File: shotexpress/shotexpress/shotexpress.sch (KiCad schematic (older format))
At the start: 16 parts

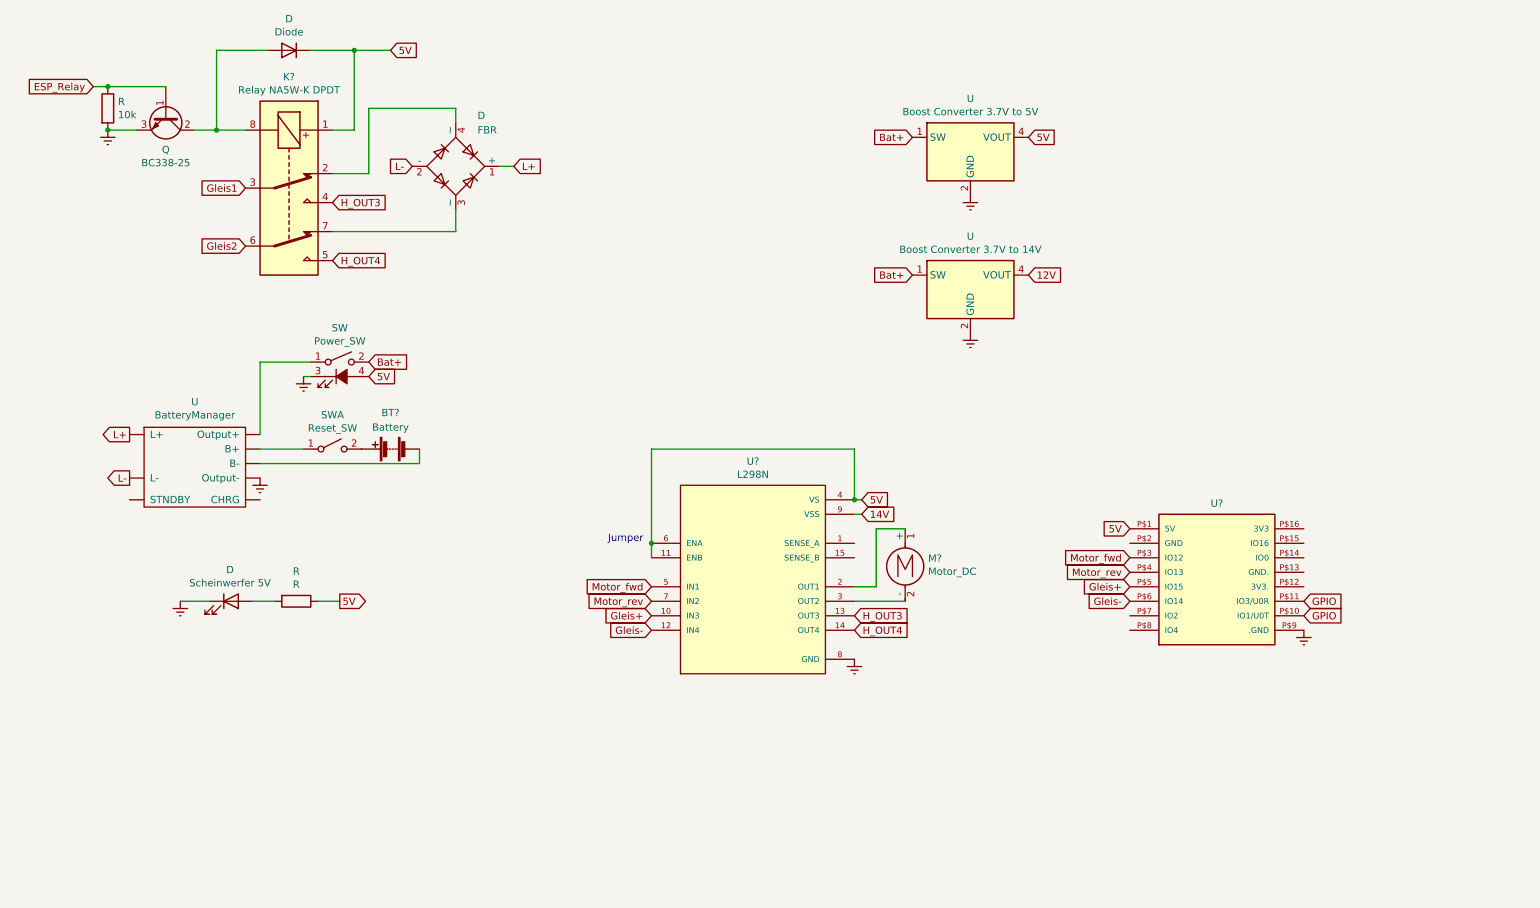
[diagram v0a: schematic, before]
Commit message: Correct kicad scheme
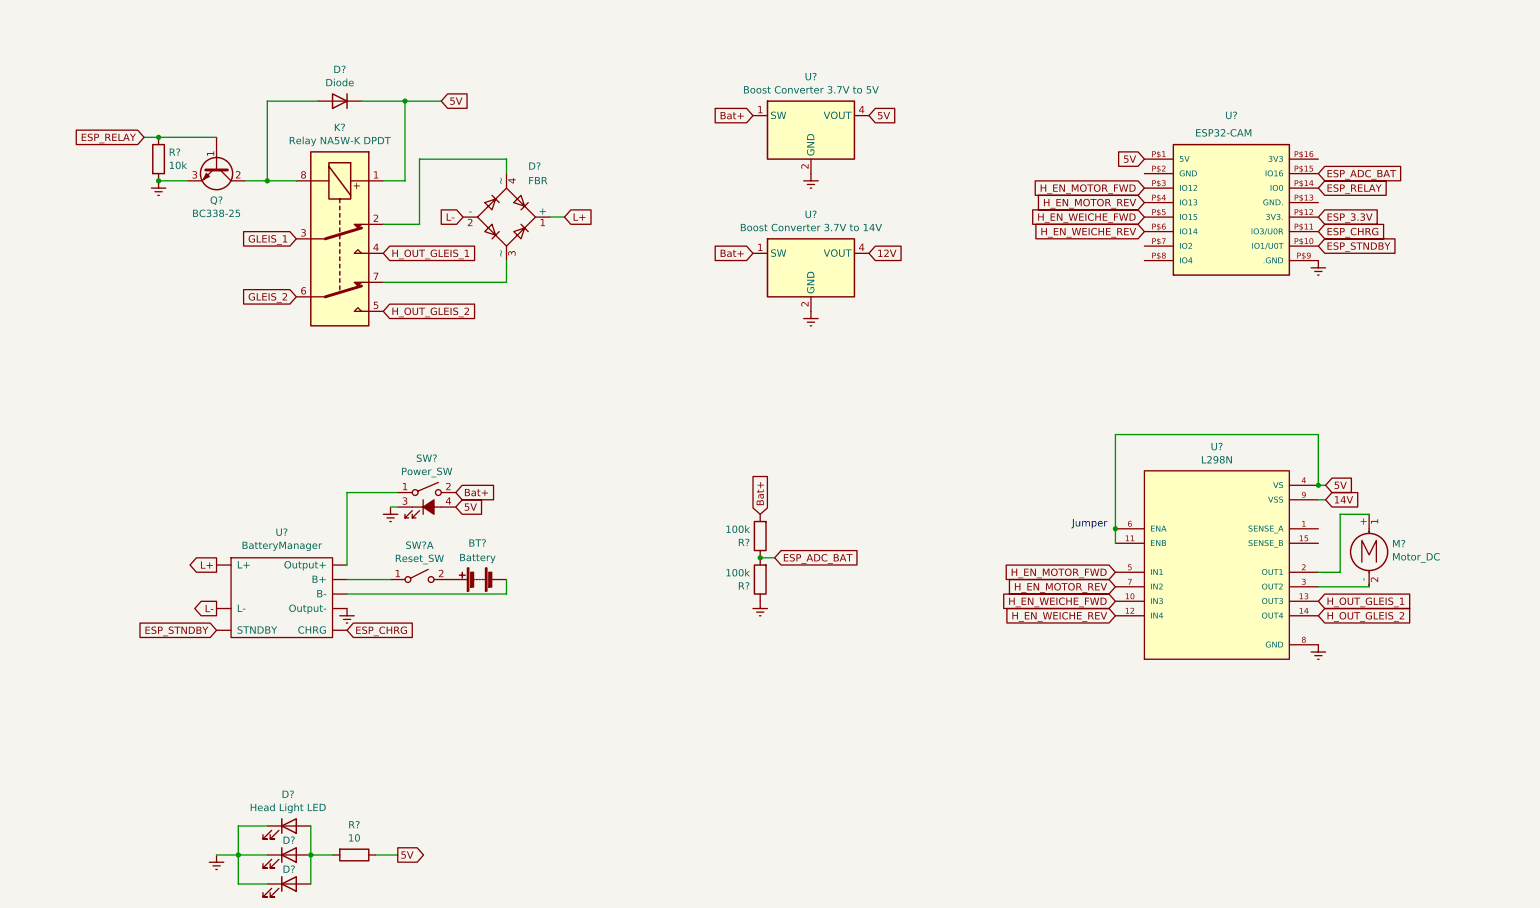
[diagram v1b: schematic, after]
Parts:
- added D? (x2): Scheinwerfer 5V, symbol Device:LED
- added R? (x2): 100k, symbol Device:R
- D?: renamed from D; value Scheinwerfer 5V -> Head Light LED
- R?: renamed from R; value R -> 10
- renumbered D to D?, Q to Q?, R to R?, SW to SW?, U to U?
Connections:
- net ESP_Relay is gone; now on net ESP_RELAY: Q?.1 (B), R?.1
- net Bat+: now also R?.2
- net Earth: now also D?.1 (K), D?.1 (K), R?.1
- net ESP_3.3V: now reaches U?.P$12 (3V3.)
- net ESP_RELAY: now reaches U?.P$14 (IO0)
- net ESP_ADC_BAT: now reaches U?.P$15 (IO16)
- net ESP_ADC_BAT: now also R?.1, R?.2
- net at D?.2 (A), R?.2: now also D?.2 (A), D?.2 (A)
- net GPIO renamed ESP_CHRG
- net ESP_CHRG: now also U?.~ (STNDBY); no longer U?.P$10 (IO1/U0T)
- net Gleis+ renamed H_EN_WEICHE_FWD
- net Gleis- renamed H_EN_WEICHE_REV
- net Gleis1 renamed GLEIS_1
- net Gleis2 renamed GLEIS_2
- net H_OUT3 renamed H_OUT_GLEIS_1
- net H_OUT4 renamed H_OUT_GLEIS_2
- net Motor_fwd renamed H_EN_MOTOR_FWD
- net Motor_rev renamed H_EN_MOTOR_REV
- new net ESP_STNDBY: U?.P$10 (IO1/U0T), U?.~ (STNDBY)
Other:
- moved on the sheet: BT?, D?, K?, M?, Q?, R?, SW?, SW?A, U?

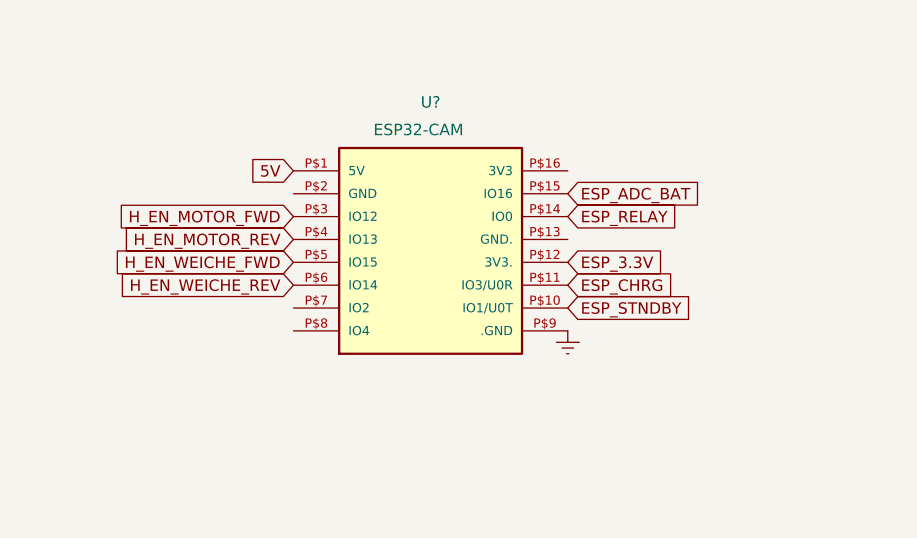
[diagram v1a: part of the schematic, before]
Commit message: Complete Kicad files
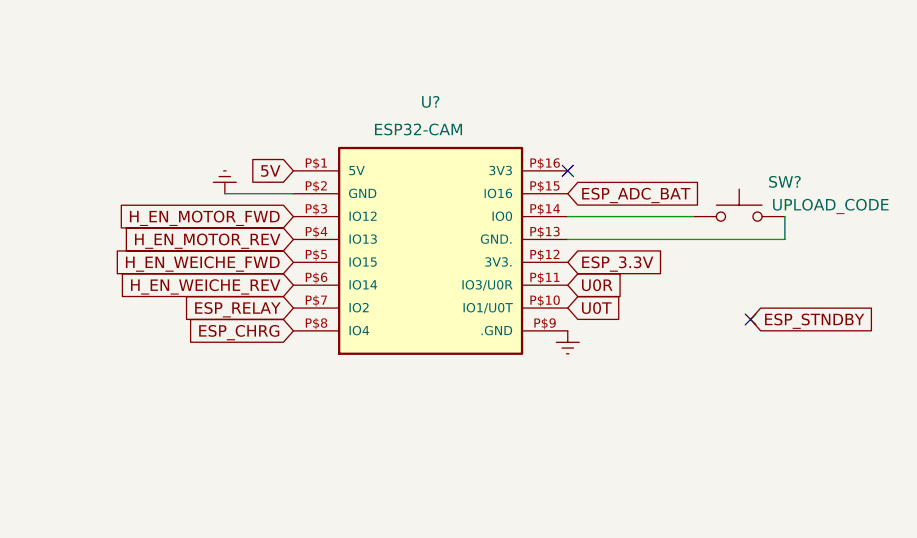
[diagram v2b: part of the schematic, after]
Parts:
- added SW?: UPLOAD_CODE, symbol Switch:SW_MEC_5G
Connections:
- net ESP_CHRG: now also U?.P$8 (IO4); no longer U?.P$11 (IO3/U0R)
- net ESP_RELAY: now also U?.P$7 (IO2); no longer U?.P$14 (IO0)
- net ESP_STNDBY: no longer U?.P$10 (IO1/U0T)
- net Earth: now also U?.P$2 (GND)
- net at U?.P$13 (GND.): now also SW?.3 (B), SW?.4 (B)
- new net: SW?.1 (A), SW?.2 (A), U?.P$14 (IO0)
- new net U0R: U?.P$11 (IO3/U0R)
- new net U0T: U?.P$10 (IO1/U0T)
- no-connect marks 0 -> 2
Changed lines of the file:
@@
 Text GLabel 6050 4650 2    50   Input ~ 0
 ESP_ADC_BAT
-Text GLabel 9800 2500 2    50   Input ~ 0
+Text GLabel 10600 2550 2    50   Input ~ 0
 ESP_STNDBY
-Text GLabel 9800 2400 2    50   Input ~ 0
+Text GLabel 8600 2600 0    50   Input ~ 0
 ESP_CHRG
-Text GLabel 9800 2100 2    50   Input ~ 0
+Text GLabel 8600 2500 0    50   Input ~ 0
 ESP_RELAY
 Text GLabel 9800 2000 2    50   Input ~ 0
@@
 Text GLabel 8400 4950 0    50   Input ~ 0
 H_EN_WEICHE_FWD
+$Comp
+L power:Earth #PWR?
+U 1 1 6115C6E3
+P 8300 2000
+F 0 "#PWR?" H 8300 1750 50  0001 C CNN
+F 1 "Earth" H 8300 1850 50  0001 C CNN
+F 2 "" H 8300 2000 50  0001 C CNN
+F 3 "~" H 8300 2000 50  0001 C CNN
+	1    8300 2000
+	-1   0    0    1
+$EndComp
+Wire Wire Line
+	8300 2000 8600 2000
+NoConn ~ 10600 2550
+Text GLabel 9800 2400 2    50   Input ~ 0
+U0R
+Text GLabel 9800 2500 2    50   Input ~ 0
+U0T
+$Comp
+L Switch:SW_MEC_5G SW?
+U 1 1 6116DAEB
+P 10550 2100
+F 0 "SW?" H 10750 2250 50  0000 C CNN
+F 1 "UPLOAD_CODE" H 10950 2150 50  0000 C CNN
+F 2 "" H 10550 2300 50  0001 C CNN
+F 3 "http://www.apem.com/int/index.php?controller=attachment&id_attachment=488" H 10550 2300 50  0001 C CNN
+	1    10550 2100
+	1    0    0    -1
+$EndComp
+Wire Wire Line
+	9800 2100 10350 2100
+Wire Wire Line
+	9800 2200 10750 2200
+Wire Wire Line
+	10750 2200 10750 2100
+NoConn ~ 9800 1900
 $EndSCHEMATC
